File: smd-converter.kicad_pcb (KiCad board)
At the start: 2 copper layers, 11.5 x 12.5 mm, 2 parts, among them J1 Conn_01x08_Male, U1 LT6234

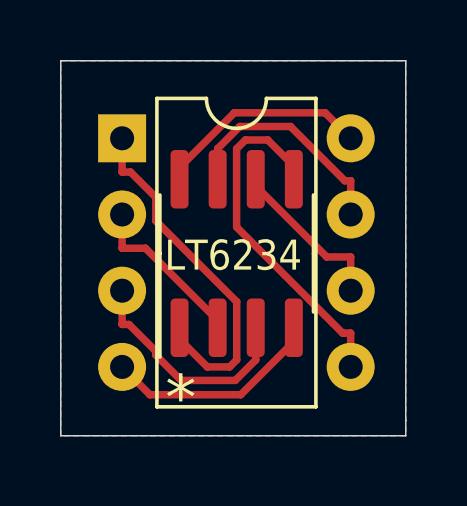
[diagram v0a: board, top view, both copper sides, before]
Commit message: Add files via upload
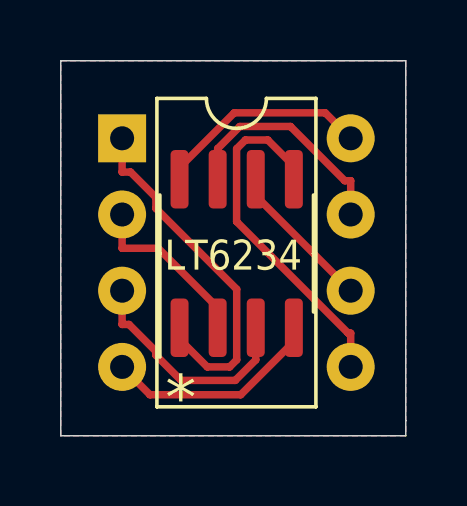
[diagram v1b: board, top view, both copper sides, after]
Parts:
- J1: footprint Package_DIP:DIP-8_W7.62mm -> tastatur:DIP-8_W7.62mm-adapter
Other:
- net class Default: clearance 0.2 -> 0.13
- rule trace_clearance: 0.2 -> 0.13
